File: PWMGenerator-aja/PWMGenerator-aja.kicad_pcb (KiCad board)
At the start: 2 copper layers, 30 parts, among them J1 Conn_01x03_Pin, J2 Barrel_Jack, Q1 2N3904, Q2 2N3904, Q3 2N3906, Q4 2N3906, SW1 SW_SPST, U1 LM7805_TO220, U2 LM339

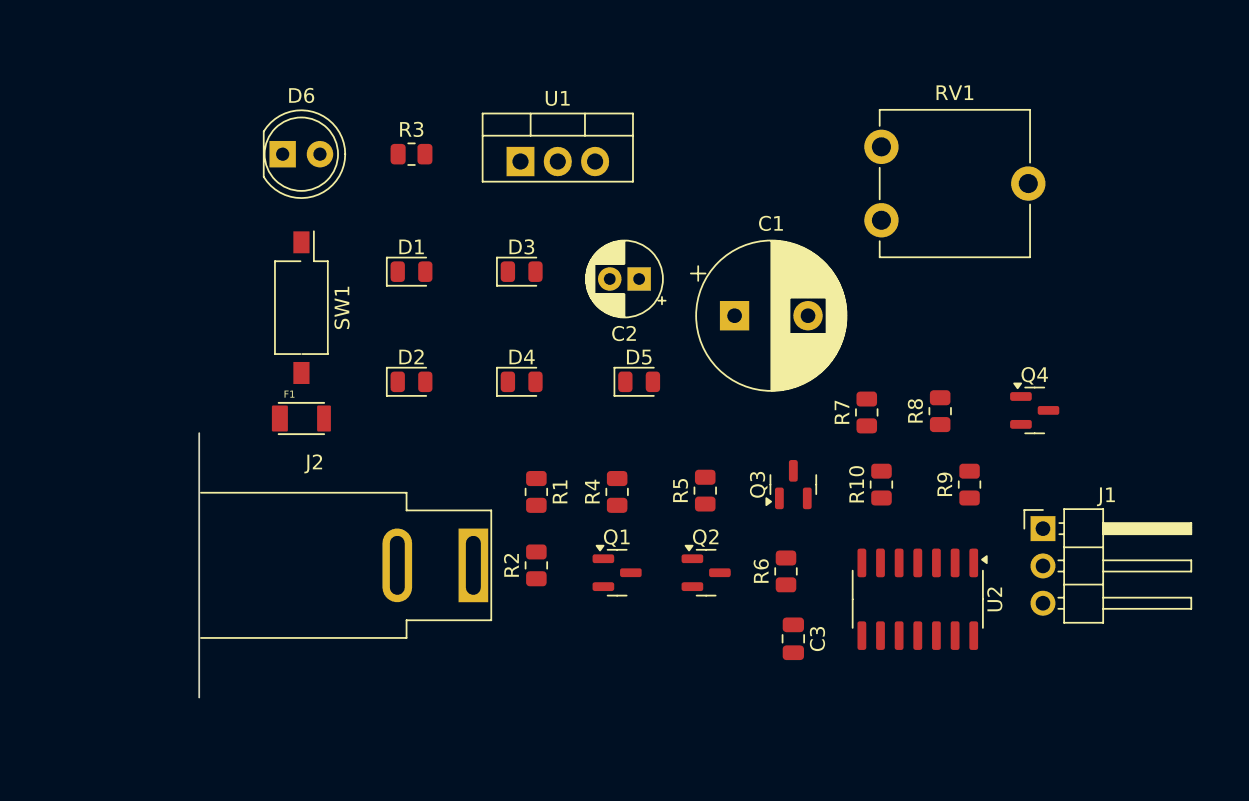
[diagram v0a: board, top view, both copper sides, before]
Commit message: bup
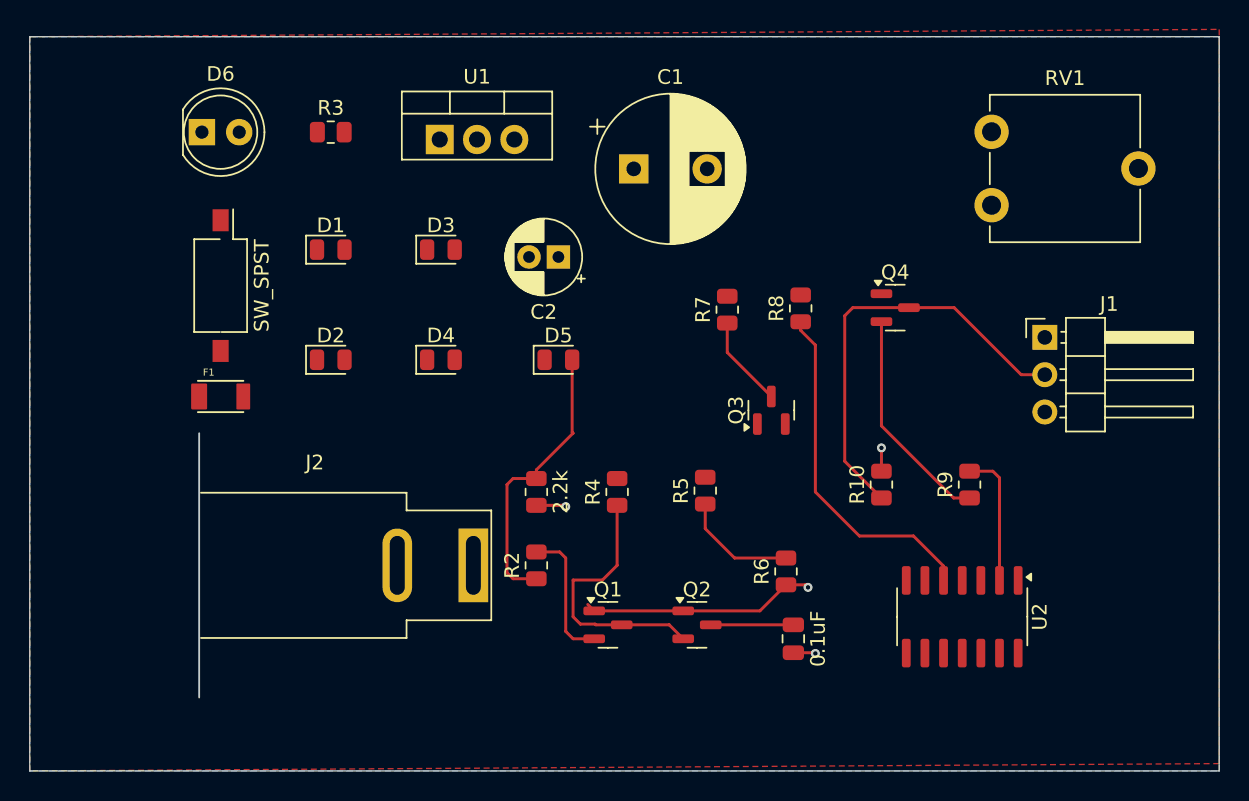
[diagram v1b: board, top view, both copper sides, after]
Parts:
- moved J1 13.0 mm to (99.1, 80.5)
- moved C1 12.1 mm to (71.1, 69.0)
- moved Q4 11.8 mm to (88.9, 78.5)
- moved R7 11.8 mm to (77.5, 78.6)
- moved R8 11.8 mm to (82.5, 78.5)
- moved RV1 7.57 mm to (95.5, 71.5)
- moved C2 5.70 mm to (66.0, 75.0)
- moved D1 5.70 mm to (50.5, 74.5)
- moved D2 5.70 mm to (50.5, 82.0)
- moved D3 5.70 mm to (58.0, 74.5)
- moved D4 5.70 mm to (58.0, 82.0)
- moved D5 5.70 mm to (66.0, 82.0)
- moved D6 5.70 mm to (41.7, 66.5)
- moved F1 5.70 mm to (43.0, 84.5)
- moved R3 5.70 mm to (50.5, 66.5)
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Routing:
- net Net-(J1-Pin_2): track 0.00 -> 29.2 mm
- net Net-(U2A-+): track 0.00 -> 23.8 mm
- net GND: track 0.00 -> 21.1 mm, vias 0 -> 4
- net Net-(D3-K): track 0.00 -> 19.6 mm
- net Net-(Q1-C): track 0.00 -> 18.1 mm
- net Net-(Q4-B): track 0.00 -> 15.1 mm
- net Net-(Q1-B): track 0.00 -> 9.32 mm
- net Net-(R9-Pad2): track 0.00 -> 9.21 mm
- net Net-(Q3-B): track 0.00 -> 8.00 mm
- net Net-(Q3-E): track 0.00 -> 6.24 mm
- net Net-(Q2-C): track 0.00 -> 5.62 mm
- added copper zone on B.Cu, net GND
- added copper zone on F.Cu, net VCC
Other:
- board outline added: 81 x 50 mm
